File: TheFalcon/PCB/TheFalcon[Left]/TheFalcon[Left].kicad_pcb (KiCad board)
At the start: 4 copper layers, 173.3 x 142.5 mm, 174 parts, among them IC1 IS31FL3729-QFLS4-TR, J1 Conn_01x01, J2 Conn_01x04_Pin, J3 Conn_01x01, J4 Conn_01x01, J5 Conn_01x01, J6 Conn_01x01, J7 Conn_01x01, SW1 SW_Push, SW2 SW_Push, U2 USBLC6-2P6, U3 USBLC6-2P6, U4 AMS1117-3.3, U6 STM32G431CBTx, Y1 X322516MOB4SI

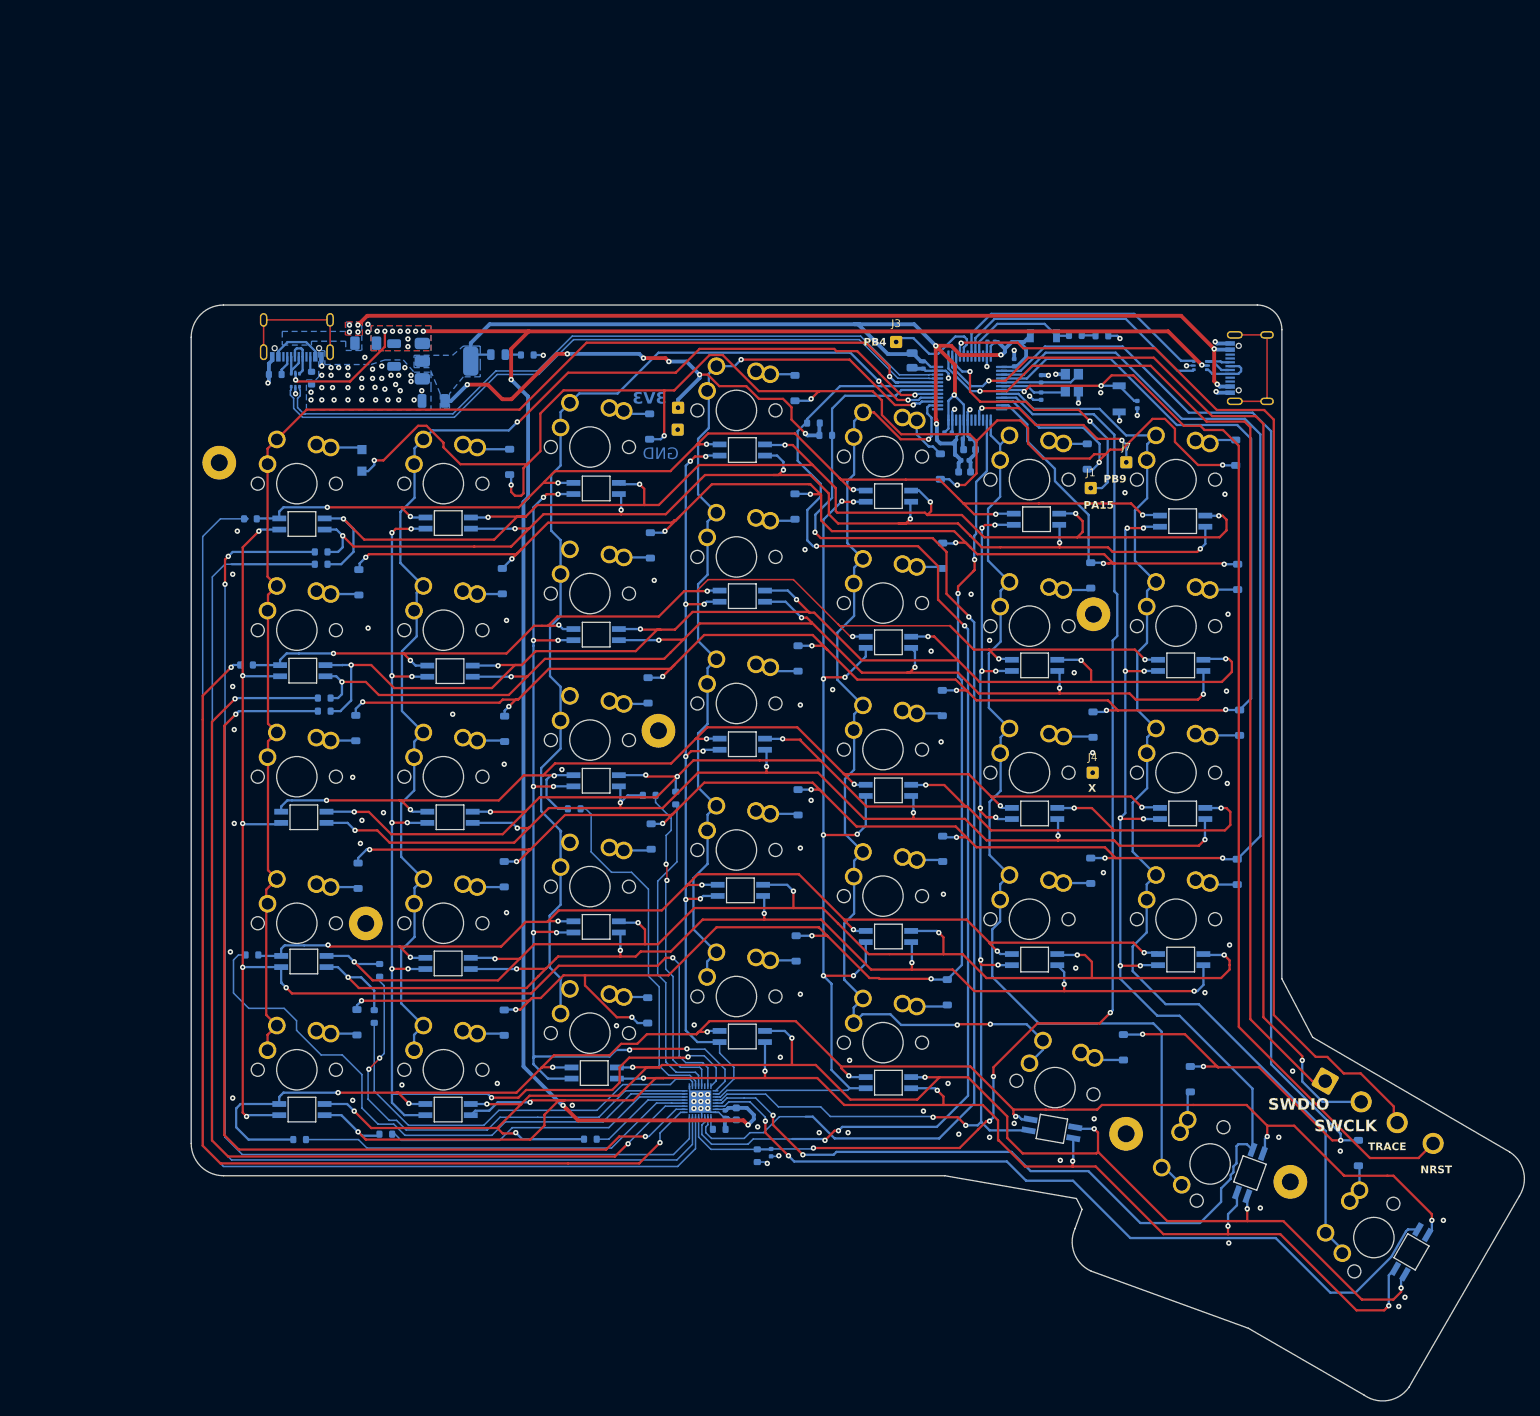
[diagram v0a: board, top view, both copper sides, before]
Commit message: Save
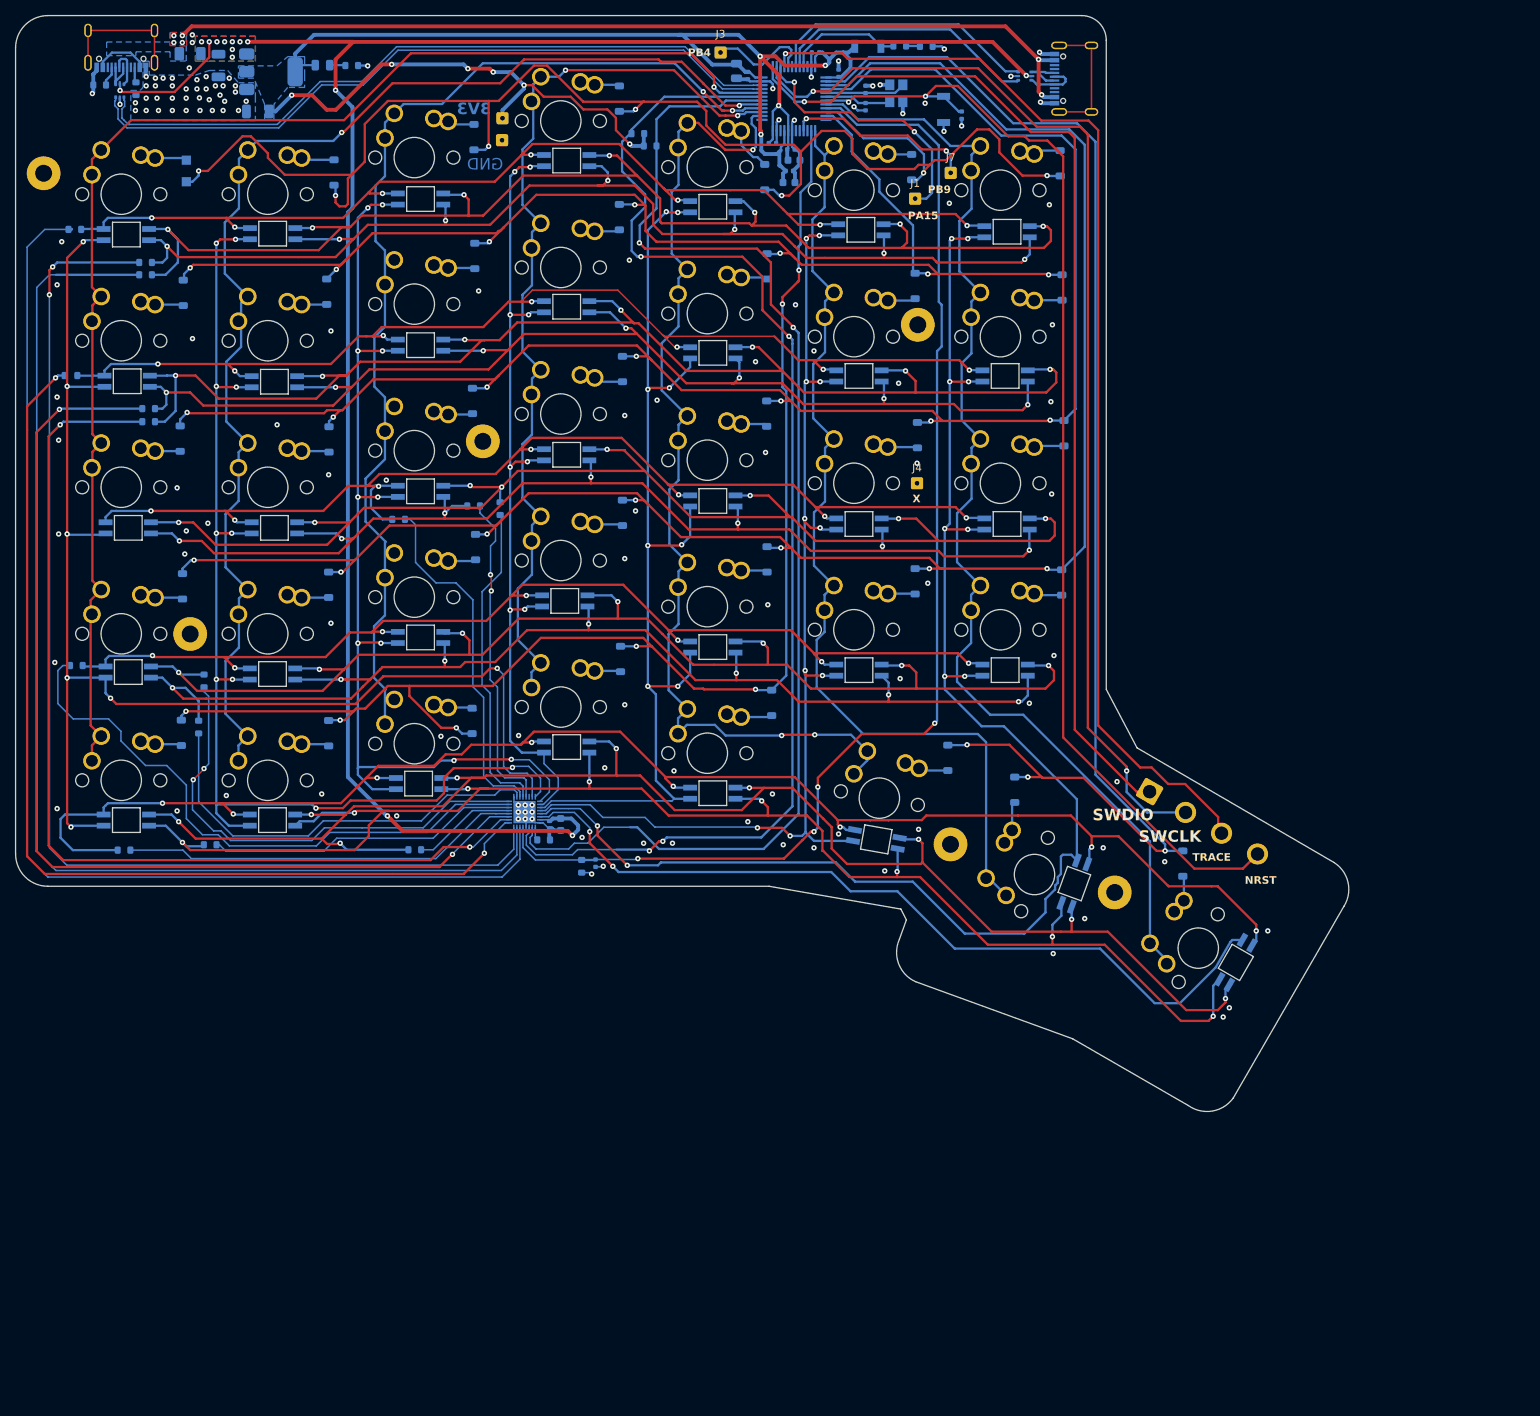
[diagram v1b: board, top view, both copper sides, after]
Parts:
- moved D36 44.0 mm to (118.0, 83.3)
- moved H1 44.0 mm to (118.3, 94.5)
- moved R23 44.0 mm to (10.9, 95.3)
- moved S13 44.0 mm to (105.8, 28.5)
- moved C11 44.0 mm to (28.3, -0.76)
- moved C12 44.0 mm to (66.2, 92.0)
- moved C7 44.0 mm to (97.3, 8.47)
- moved D24 44.0 mm to (56.6, 55.9)
- moved D27 44.0 mm to (113.7, 60.3)
- moved D29 44.0 mm to (18.3, 80.0)
- moved D3 44.0 mm to (56.4, 2.57)
- moved D30 44.0 mm to (37.5, 80.1)
- moved D38 44.0 mm to (148.5, 97.0)
- moved H4 44.0 mm to (139.7, 100.8)
- moved J1 44.0 mm to (113.7, 10.6)
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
